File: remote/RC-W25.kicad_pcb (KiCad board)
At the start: 2 copper layers, 36 x 100.1 mm, 56 parts, among them J1 USB_C_Receptacle_USB2.0_14P, P1 JST CONN, P2 JST CONN, Q1 NMOS, SW1 Button, SW2 Button, SW3 YTSPS-22E58LM, SW4 Button, U1 ESP32-C6-MINI-1, U2 MCP73831-5-OT, U3 AP62300Z6, U4 TMAG5253

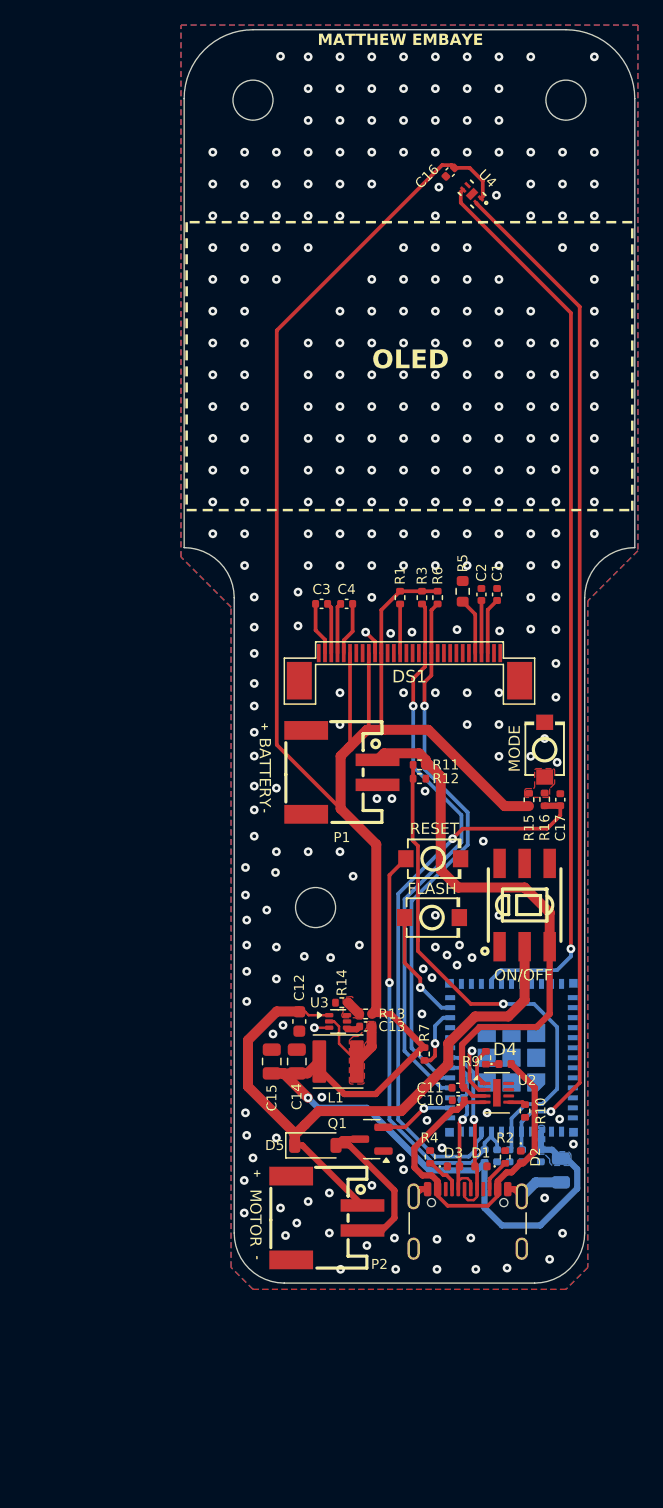
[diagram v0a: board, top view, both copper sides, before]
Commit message: CRC V3
V 3.0.0
Initial version of CRC V3, fully redesigned remote
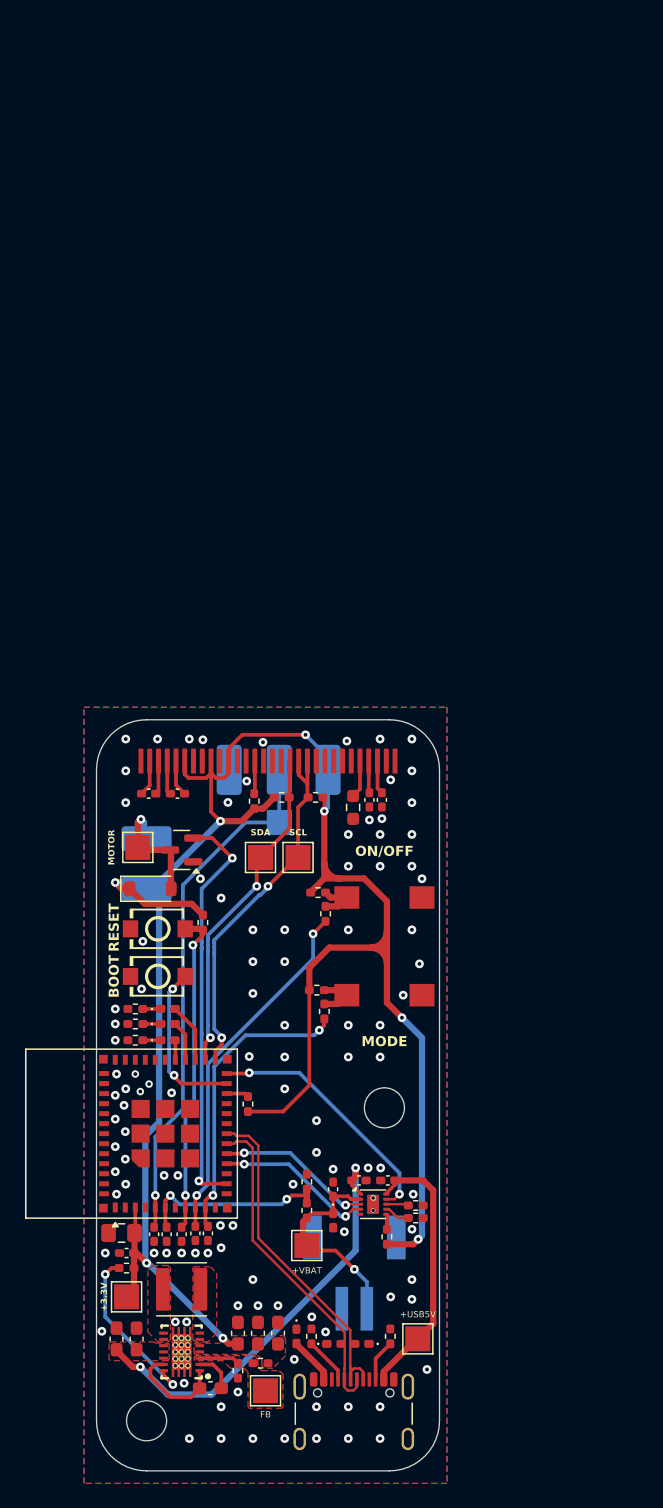
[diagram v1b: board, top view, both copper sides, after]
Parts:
- removed G***: LOGO, LOGO
- removed H3: MountingHole, MountingHole:MountingHole_3.2mm_M3
- removed P1, P2: JST CONN, footprints:CONN-SMD_2P-P2.00_XUNPU_WAFER-PH2.0-2PWB
- removed SW1, SW2, SW4: Button, footprints:SW-SMD_L3.9-W3.0-P4.45
- removed SW3: YTSPS-22E58LM, footprints:SW-SMD_6P-YTSPS-22E58LM
- removed U4: TMAG5253, footprints:X2SON4_DMR_TEX
- added +3.3V: TEST POINT, TestPoint:TestPoint_Pad_2.0x2.0mm, F.Cu at (102.4, 126.1)
- added +USB5V: TEST POINT, TestPoint:TestPoint_Pad_2.0x2.0mm, F.Cu at (125.7, 129.5)
- added +VBAT: TEST POINT, TestPoint:TestPoint_Pad_2.0x2.0mm, F.Cu at (116.8, 122.0)
- added BATTERY: JST CONN, footprints:CONN-SMD_2P-P2.00_XUNPU_WAFER-PH2.0-2PWB, B.Cu at (120.6, 124.2)
- added BOOT: Button, footprints:SW-SMD_L3.9-W3.0-P4.45, F.Cu at (104.9, 100.5)
- added C18: 10uF, Capacitor_SMD:C_0402_1005Metric_Pad0.74x0.62mm_HandSolder, F.Cu at (121.0, 116.8)
- added C19: 100nF, Capacitor_SMD:C_0402_1005Metric_Pad0.74x0.62mm_HandSolder, F.Cu at (108.9, 121.0)
- added C20: 100nF, Capacitor_SMD:C_0402_1005Metric_Pad0.74x0.62mm_HandSolder, F.Cu at (107.9, 121.0)
- added D6: GLED, Diode_SMD:D_0402_1005Metric_Pad0.77x0.64mm_HandSolder, F.Cu at (105.7, 105.6)
- added D7: ZENER 5V, Diode_SMD:D_0402_1005Metric_Pad0.77x0.64mm_HandSolder, F.Cu at (118.9, 120.0)
- added D8: D_Schottky, Diode_SMD:D_SOD-123, F.Cu at (104.3, 93.5)
- added FB: TEST POINT, TestPoint:TestPoint_Pad_2.0x2.0mm, F.Cu at (113.5, 133.6)
- added JOYSTICK: TEST POINT, TestPoint:TestPoint_Pad_2.0x2.0mm, B.Cu at (114.6, 88.2)
- added JOYSTICK: JOYSTICK, footprints:Joystick Potentiometer Pads, B.Cu at (114.6, 84.0)
- added MODE: Button, footprints:Box Tactile Button Switch, F.Cu at (123.0, 102.0)
- added MOTOR: TEST POINT, TestPoint:TestPoint_Pad_2.0x2.0mm, F.Cu at (103.3, 90.2)
- added MOTOR: MOTOR, footprints:Motor Pads, B.Cu at (104.0, 91.5)
- added ON/OFF: Button, footprints:Box Tactile Button Switch, F.Cu at (123.0, 94.2)
- added R17: 1k, Resistor_SMD:R_0402_1005Metric_Pad0.72x0.64mm_HandSolder, F.Cu at (116.8, 119.2)
- added R18: 3.7k, Resistor_SMD:R_0402_1005Metric_Pad0.72x0.64mm_HandSolder, F.Cu at (116.8, 116.9)
- added R19: 1M, Resistor_SMD:R_0402_1005Metric_Pad0.72x0.64mm_HandSolder, F.Cu at (102.4, 123.8)
- added R20: 10k, Resistor_SMD:R_0402_1005Metric_Pad0.72x0.64mm_HandSolder, F.Cu at (117.6, 101.6)
- added R21: 10k, Resistor_SMD:R_0402_1005Metric_Pad0.72x0.64mm_HandSolder, F.Cu at (117.7, 93.8)
- added R22: 10k, Resistor_SMD:R_0402_1005Metric_Pad0.72x0.64mm_HandSolder, F.Cu at (118.2, 103.3)
- added R23: 10k, Resistor_SMD:R_0402_1005Metric_Pad0.72x0.64mm_HandSolder, F.Cu at (118.3, 95.5)
- added RESET: Button, footprints:SW-SMD_L3.9-W3.0-P4.45, F.Cu at (104.9, 96.7)
- added SCL: TEST POINT, TestPoint:TestPoint_Pad_2.0x2.0mm, F.Cu at (116.1, 91.0)
- added SDA: TEST POINT, TestPoint:TestPoint_Pad_2.0x2.0mm, F.Cu at (113.1, 91.0)
- C1: value 2.2uF -> 4.7uF; footprint Capacitor_SMD:C_0402_1005Metric -> Capacitor_SMD:C_0402_1005Metric_Pad0.74x0.62mm_HandSolder
- C10, C3, C4: footprint Capacitor_SMD:C_0402_1005Metric -> Capacitor_SMD:C_0402_1005Metric_Pad0.74x0.62mm_HandSolder
- C11: value 4.7uF -> 10uF; footprint Capacitor_SMD:C_0402_1005Metric -> Capacitor_SMD:C_0603_1608Metric_Pad1.08x0.95mm_HandSolder
- C12: footprint Capacitor_SMD:C_0603_1608Metric -> Capacitor_SMD:C_0603_1608Metric_Pad1.08x0.95mm_HandSolder
- C13: footprint Capacitor_SMD:C_0402_1005Metric -> Capacitor_SMD:C_0603_1608Metric_Pad1.08x0.95mm_HandSolder
- C14: value 22uF -> 1uF; footprint Capacitor_SMD:C_0805_2012Metric -> Capacitor_SMD:C_0402_1005Metric_Pad0.74x0.62mm_HandSolder
- C15: footprint Capacitor_SMD:C_0805_2012Metric -> Capacitor_SMD:C_0603_1608Metric_Pad1.08x0.95mm_HandSolder
- C16, C17: value 100nF -> 22uF; footprint Capacitor_SMD:C_0402_1005Metric -> Capacitor_SMD:C_0603_1608Metric_Pad1.08x0.95mm_HandSolder
- C2: value 2.2uF -> 10uF; footprint Capacitor_SMD:C_0402_1005Metric -> Capacitor_SMD:C_0402_1005Metric_Pad0.74x0.62mm_HandSolder
- C5, C6, C7, C9: footprint Capacitor_SMD:C_0402_1005Metric -> Capacitor_SMD:C_0402_1005Metric_Pad0.74x0.62mm_HandSolder; moved to F.Cu
- C8: footprint Capacitor_SMD:C_0805_2012Metric -> Capacitor_SMD:C_0805_2012Metric_Pad1.18x1.45mm_HandSolder; moved to F.Cu
- D1, D2, D3: footprint footprints:D_0402_1005Metric -> Diode_SMD:D_0402_1005Metric_Pad0.77x0.64mm_HandSolder
- D4: value LED -> RLED; footprint footprints:D_0402_1005Metric -> Diode_SMD:D_0402_1005Metric_Pad0.77x0.64mm_HandSolder
- D5: value D_Schottky -> ORLED; footprint Diode_SMD:D_SOD-123 -> Diode_SMD:D_0402_1005Metric_Pad0.77x0.64mm_HandSolder
- DS1: value FPC 0.5mm 30P -> FPC 0.7mm 30P; footprint footprints:FPC-30P-0.5mm -> footprints:FPC 0.7mm 30P
- L1: value 3.3uH -> 1.5uH
- R1: value 4.7k -> 390k; footprint Resistor_SMD:R_0402_1005Metric -> Resistor_SMD:R_0603_1608Metric_Pad0.98x0.95mm_HandSolder
- R10: value 2k -> 300; footprint Resistor_SMD:R_0402_1005Metric -> Resistor_SMD:R_0402_1005Metric_Pad0.72x0.64mm_HandSolder
- R11, R3, R7: footprint Resistor_SMD:R_0402_1005Metric -> Resistor_SMD:R_0402_1005Metric_Pad0.72x0.64mm_HandSolder
- R12: value 1.1k -> 5k; footprint Resistor_SMD:R_0402_1005Metric -> Resistor_SMD:R_0402_1005Metric_Pad0.72x0.64mm_HandSolder
- R13: value 31.6k -> 1k; footprint Resistor_SMD:R_0402_1005Metric -> Resistor_SMD:R_0402_1005Metric_Pad0.72x0.64mm_HandSolder
- R14: value 10k -> 1k; footprint Resistor_SMD:R_0402_1005Metric -> Resistor_SMD:R_0402_1005Metric_Pad0.72x0.64mm_HandSolder
- R15: value 10k -> 1M; footprint Resistor_SMD:R_0402_1005Metric -> Resistor_SMD:R_0402_1005Metric_Pad0.72x0.64mm_HandSolder
- R16: value 10k -> 180k; footprint Resistor_SMD:R_0402_1005Metric -> Resistor_SMD:R_0402_1005Metric_Pad0.72x0.64mm_HandSolder
- R2, R4: value 5.1k -> 4.7k; footprint Resistor_SMD:R_0402_1005Metric -> Resistor_SMD:R_0402_1005Metric_Pad0.72x0.64mm_HandSolder
- R5: value 390k -> 5.1k; footprint Resistor_SMD:R_0603_1608Metric -> Resistor_SMD:R_0402_1005Metric_Pad0.72x0.64mm_HandSolder
- R6: value 4.7k -> 5.1k; footprint Resistor_SMD:R_0402_1005Metric -> Resistor_SMD:R_0402_1005Metric_Pad0.72x0.64mm_HandSolder
- R8: footprint Resistor_SMD:R_0402_1005Metric -> Resistor_SMD:R_0402_1005Metric_Pad0.72x0.64mm_HandSolder; moved to F.Cu
- R9: value 470 -> 300; footprint Resistor_SMD:R_0402_1005Metric -> Resistor_SMD:R_0402_1005Metric_Pad0.72x0.64mm_HandSolder
- U1: moved to F.Cu
- U2: value MCP73831-5-OT -> BQ25185; footprint Package_DFN_QFN:DFN-8-1EP_2x3mm_P0.5mm_EP0.61x2.2mm -> footprints:WSON-10 BQ25185
- U3: value AP62300Z6 -> TPS63020; footprint Package_TO_SOT_SMD:SOT-563 -> footprints:TPS63020_VSON(14)
- moved H2 105.8 mm to (104.0, 136.0)
- moved C16 94.0 mm to (112.9, 129.0), turned to 90 degrees
- moved H1 81.8 mm to (123.0, 111.0)
- moved R6 59.9 mm to (117.2, 129.3), turned to 90 degrees
- moved R5 59.8 mm to (123.5, 129.3)
- moved R16 51.8 mm to (111.3, 132.0)
- moved R15 49.9 mm to (113.1, 131.4), turned to 180 degrees
- moved C17 48.2 mm to (114.5, 129.0)
- moved C8 35.5 mm to (102.0, 121.0), turned to 180 degrees
- moved R12 35.1 mm to (125.5, 119.8)
- moved C9 34.0 mm to (102.4, 122.6), turned to 180 degrees
- moved C11 33.9 mm to (101.6, 129.5), turned to 90 degrees
- moved R2 33.8 mm to (114.8, 86.2), turned to 0 degrees
- moved R10 31.9 mm to (103.1, 104.3), turned to 180 degrees
- moved R11 31.6 mm to (103.1, 105.6)
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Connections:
- net ADC_HALLEFFECT1 renamed ADC_JOYSTICK
- C1 pad 1: Net-(DS1-VDisplay) -> Net-(DS1-VCOMH)
- C11 pad 1: Net-(P1-Pin_1) -> +VSYS
- C12 pad 1: +VBAT -> +VSYS
- C13 pad 1: Net-(U3-SW) -> Net-(U3-PS/SYNC)
- C13 pad 2: Net-(U3-BST) -> GND
- C14 pad 1: +3.3V -> +VBAT
- C17 pad 1: GPIO_MODE -> +3.3V
- C2 pad 1: Net-(DS1-VCOMH) -> Net-(DS1-VDisplay)
- C6 pad 1: /RC_Connections/RESET -> ADC_BATTERYPERCENT
- C7 pad 1: ADC_BATTERYPERCENT -> /Connections/RESET
- D4 pad 2: +USB5V -> Net-(D4-A)
- D5 pad 1: +VBAT -> Net-(D5-K)
- DS1 pad 20: unconnected-(DS1-D2-Pad20) -> SCL_DISPLAY
- DS1 pad 7: GND -> unconnected-(DS1-N.C.-Pad7)
- L1 pad 1: Net-(U3-SW) -> Net-(L1-Pad1)
- L1 pad 2: +3.3V -> Net-(L1-Pad2)
- Q1 pad 3: Net-(D5-A) -> Net-(D8-A)
- R1 pad 1: +3.3V -> Net-(DS1-IREF)
- R1 pad 2: Net-(DS1-Reset) -> GND
- R10 pad 1: Net-(U2-PROG) -> Net-(D5-K)
- R11 pad 1: Net-(P1-Pin_1) -> Net-(D6-K)
- R11 pad 2: ADC_BATTERYPERCENT -> GND
- R12 pad 1: ADC_BATTERYPERCENT -> /Power/ILIM/VSET
- R13 pad 1: +3.3V -> Net-(U2-ISET)
- R13 pad 2: Net-(U3-FB) -> GND
- R14 pad 1: Net-(U3-FB) -> +3.3V
- R14 pad 2: GND -> /Power/TS/MR
- R15 pad 2: Net-(R15-Pad2) -> Net-(U3-FB)
- R16 pad 1: Net-(R15-Pad2) -> Net-(U3-FB)
- R16 pad 2: GPIO_MODE -> GND
- R2 pad 1: Net-(J1-CC2) -> +3.3V
- R2 pad 2: GND -> SDA_DISPLAY
- R3 pad 2: SDA_DISPLAY -> Net-(DS1-Reset)
- R4 pad 1: Net-(J1-CC1) -> +3.3V
- R4 pad 2: GND -> SCL_DISPLAY
- R5 pad 1: Net-(DS1-IREF) -> Net-(J1-CC2)
- R6 pad 1: +3.3V -> Net-(J1-CC1)
- R6 pad 2: SCL_DISPLAY -> GND
- R8 pad 2: /RC_Connections/RESET -> /Connections/RESET
- R9 pad 2: Net-(U2-STAT) -> GND
- U1 pad 10: unconnected-(U1-IO5-Pad10) -> GPIO_MODE
- U1 pad 15: SDA_DISPLAY -> CH_EN
- U1 pad 16: SCL_DISPLAY -> CHSTAT2
- U1 pad 23: /RC_Connections/FLASH -> /Connections/FLASH
- U1 pad 24: unconnected-(U1-IO18-Pad24) -> CHSTAT1
- U1 pad 25: unconnected-(U1-IO19-Pad25) -> SCL_DISPLAY
- U1 pad 26: unconnected-(U1-IO20-Pad26) -> SDA_DISPLAY
- U1 pad 27: unconnected-(U1-IO21-Pad27) -> Net-(D4-A)
- U1 pad 28: GPIO_EN1 -> Net-(D5-A)
- U1 pad 29: unconnected-(U1-IO23-Pad29) -> Net-(D6-A)
- U1 pad 8: /RC_Connections/RESET -> /Connections/RESET
- U1 pad 9: GPIO_MODE -> ON/OFF
- U2 pad 1: Net-(U2-STAT) -> +VSYS
- U2 pad 2: GND -> +VBAT
- U2 pad 3: Net-(P1-Pin_1) -> CHSTAT2
- U2 pad 4: +USB5V -> CH_EN
- U2 pad 5: Net-(U2-PROG) -> GND
- U2 pad 6: (no net) -> /Power/TS/MR
- U2 pad 7: (no net) -> /Power/ILIM/VSET
- U2 pad 8: (no net) -> Net-(U2-ISET)
- U2 pad 9: (no net) -> CHSTAT1
- U3 pad 1: +VBAT -> Net-(U3-PS/SYNC)
- U3 pad 2: Net-(U3-SW) -> GND
- U3 pad 3: GND -> Net-(U3-FB)
- U3 pad 4: Net-(U3-BST) -> +3.3V
- U3 pad 5: unconnected-(U3-EN-Pad5) -> +3.3V
- U3 pad 6: Net-(U3-FB) -> Net-(L1-Pad2)
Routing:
- net GPIO_EN1: track 72.4 -> 0.00 mm, vias 1 -> 0
- net Net-(P1-Pin_1): track 45.4 -> 0.00 mm
- net ADC_JOYSTICK: track 81.9 -> 42.3 mm
- net +VBAT: track 54.2 -> 16.7 mm, vias 0 -> 1
- net +VSYS: track 0.00 -> 34.4 mm, vias 0 -> 2
- net /RC_Connections/RESET: track 34.2 -> 0.00 mm, vias 1 -> 0
- net ON/OFF: track 0.00 -> 28.7 mm, vias 0 -> 2
- net GPIO_RUMBLE_CNTL: track 5.97 -> 33.0 mm, vias 1 -> 2
- net +3.3V: track 193.8 -> 167.0 mm, vias 1 -> 8
- net /Connections/RESET: track 0.00 -> 26.2 mm, vias 0 -> 2
- net ADC_BATTERYPERCENT: track 40.8 -> 15.3 mm, vias 1 -> 2
- net GPIO_MODE: track 45.0 -> 24.1 mm, vias 1 -> 2
- net CHSTAT1: track 0.00 -> 20.1 mm, vias 0 -> 2
- net SDA_DISPLAY: track 44.6 -> 26.8 mm, vias 1 -> 2
- net Net-(U3-PG): track 0.00 -> 13.8 mm, vias 0 -> 2
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- added copper zone on F.Cu, net +3.3V
- added copper zone on F.Cu, net +VSYS
- added copper zone on F.Cu, net Net-(L1-Pad1)
- added copper zone on F.Cu, net Net-(L1-Pad2)
- removed copper zone on B.Cu, net +3.3V
- removed copper zone on F.Cu, net Net-(R15-Pad2)
- removed copper zone on F.Cu, net Net-(U3-SW)
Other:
- board size 36 x 100.1 mm -> 27.4 x 60 mm
- board text removed: "+"
- board text removed: "-"
- board text removed: "BATTERY"
- board text removed: "FLASH"
- board text removed: "MATTHEW EMBAYE"
- board text removed: "MODE"
- board text removed: "MOTOR"
- board text removed: "OLED"
- board text removed: "ON/OFF"
- board text removed: "RESET"
